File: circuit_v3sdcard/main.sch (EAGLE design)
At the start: 24 parts, among them CN1 SD, CN3 MICROSD, CN4 5035481020, IC1 C8051F381-GM, IC3 N25Q512A, IC4 KC2016K, IC6 MPU-9250

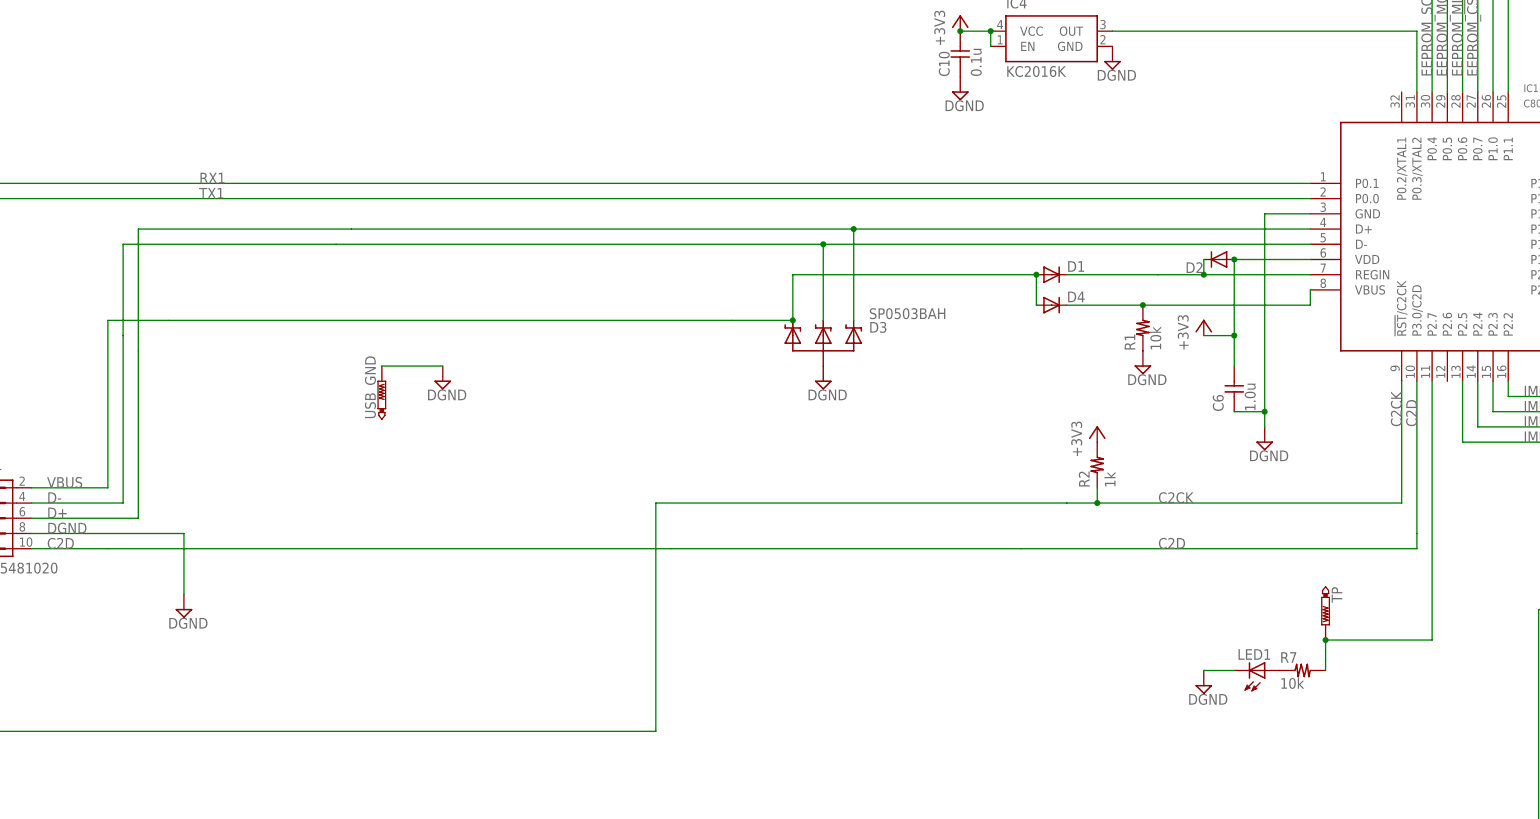
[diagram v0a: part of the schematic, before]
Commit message: Modified v3 circuit
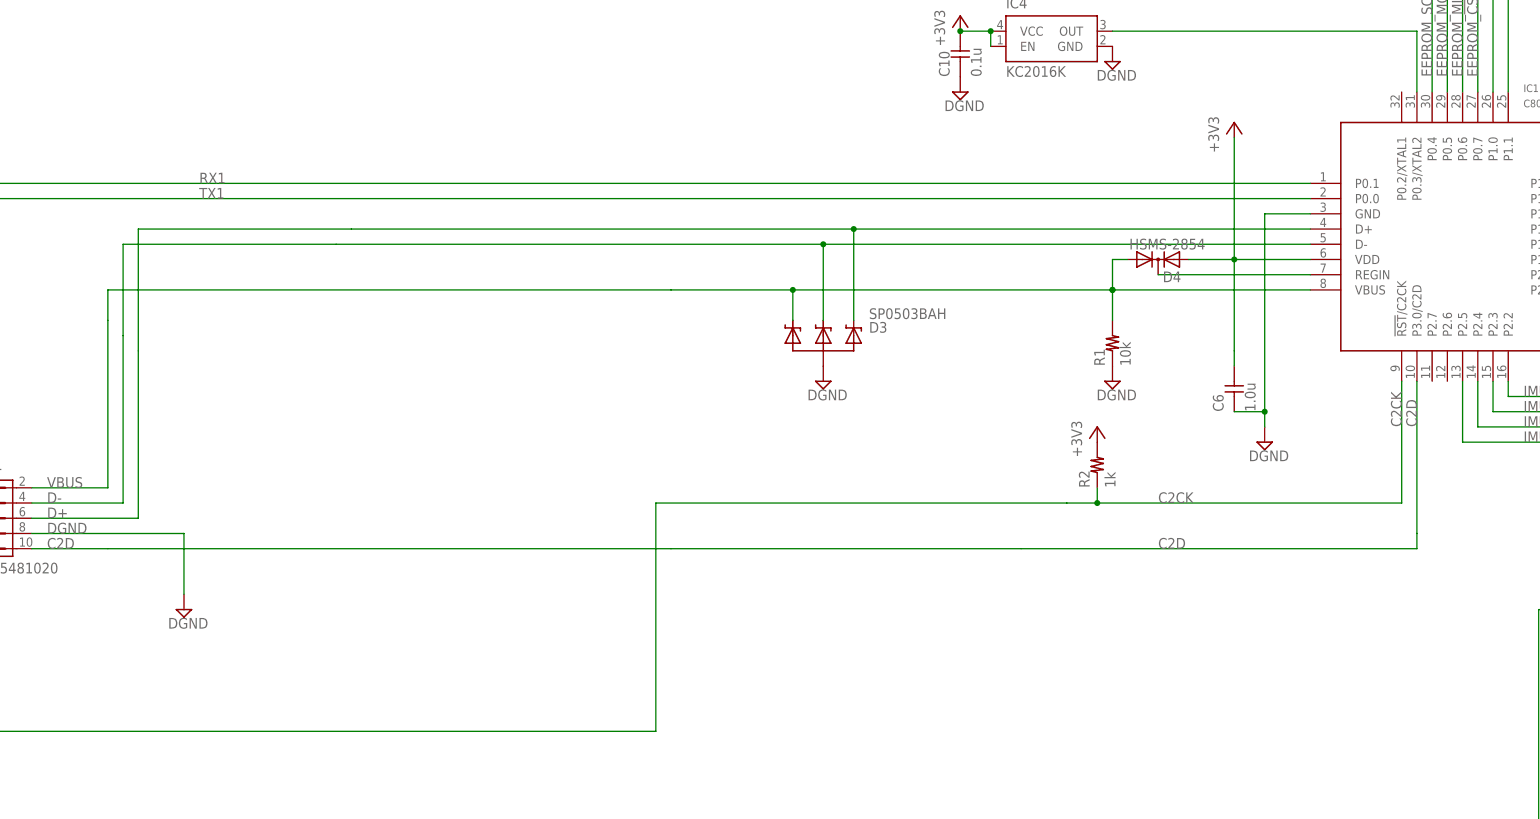
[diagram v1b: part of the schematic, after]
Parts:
- removed D1, D2: (no value), diode:DIODE-SOD323-W
- removed LED1: (no value), LED:LED1608O
- removed R7: 10k, reg,cap:R-1005
- removed TP: PTR1TP10R, testpad:PTR1TP10R
- removed USB_GND: PTR1TP11R, testpad:PTR1TP11R
- D4: value (none) -> HSMS-2854; device diode:DIODE-SOD323-W -> avago:HSMS-2854
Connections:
- removed net N$15: IC1G$1.P2.7, R7.P$2, TP.TP
- removed net N$4: D1.C, D2.C, IC1G$1.REGIN
- removed net N$5: D4.C, IC1G$1.VBUS, R1.P$2
- removed net N$9: LED1.A, R7.P$1
- new net N$1: D4.C, IC1G$1.REGIN
- net +3V3: now also D4.A2; no longer D2.A
- net DGND: no longer LED1.K, USB_GND.TP
- net VBUS: now also D4.A1, IC1G$1.VBUS, R1.P$2; no longer D1.A, D4.A
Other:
- moved on the sheet: R1
